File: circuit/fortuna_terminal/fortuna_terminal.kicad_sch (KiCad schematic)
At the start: 14 parts

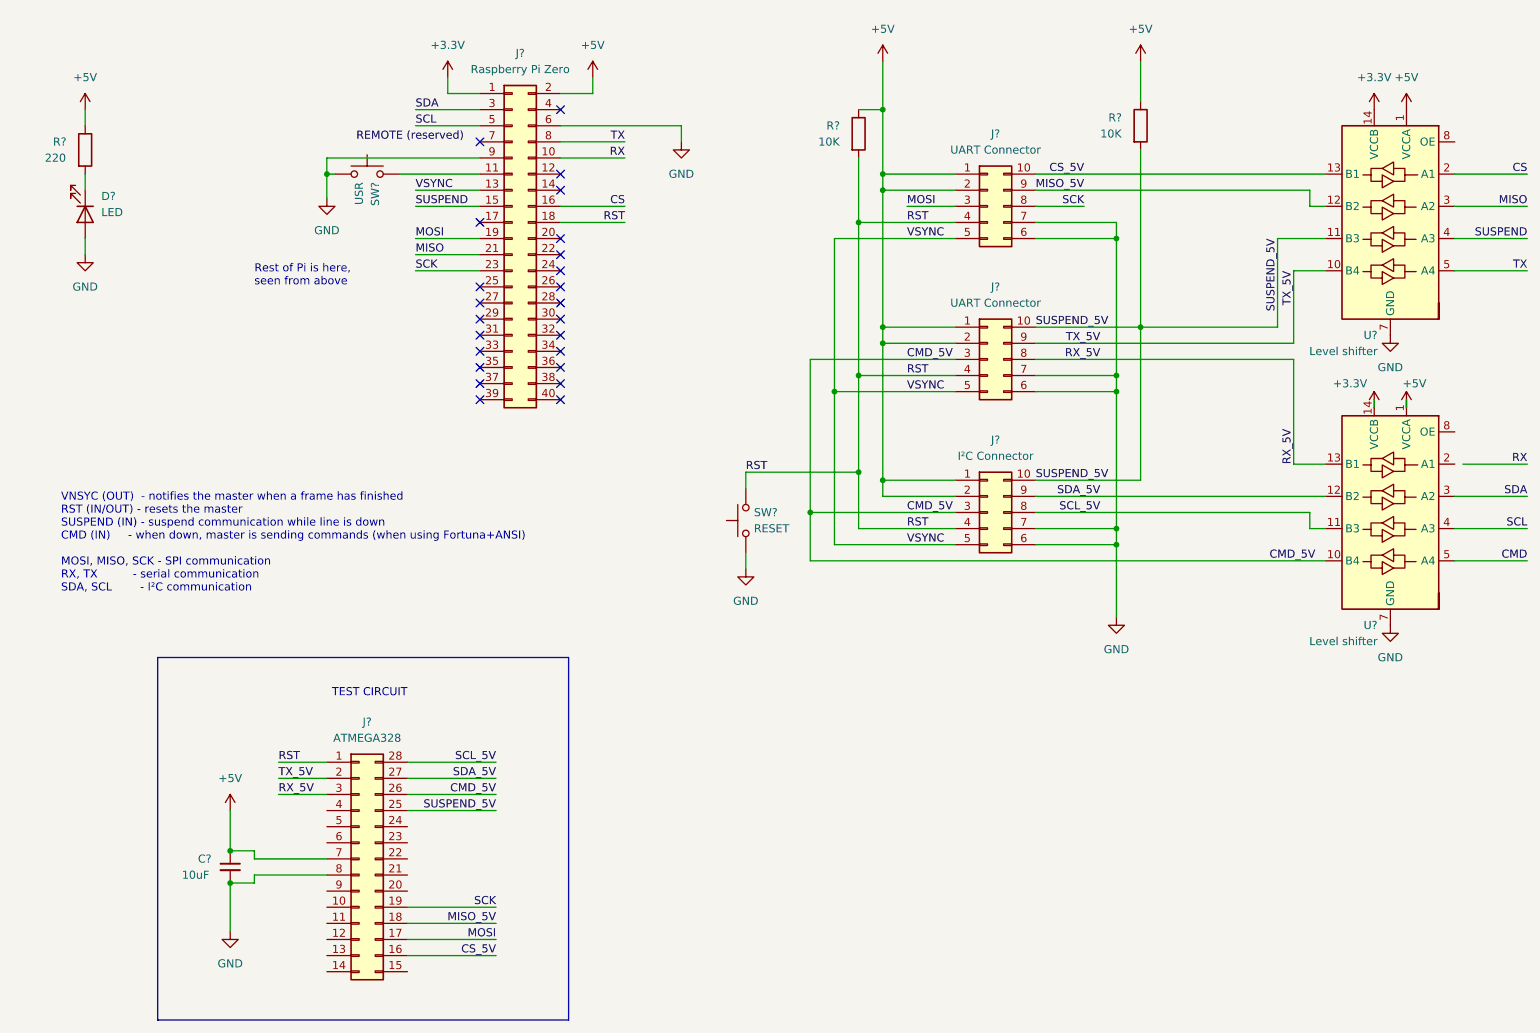
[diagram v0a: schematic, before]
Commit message: WIP
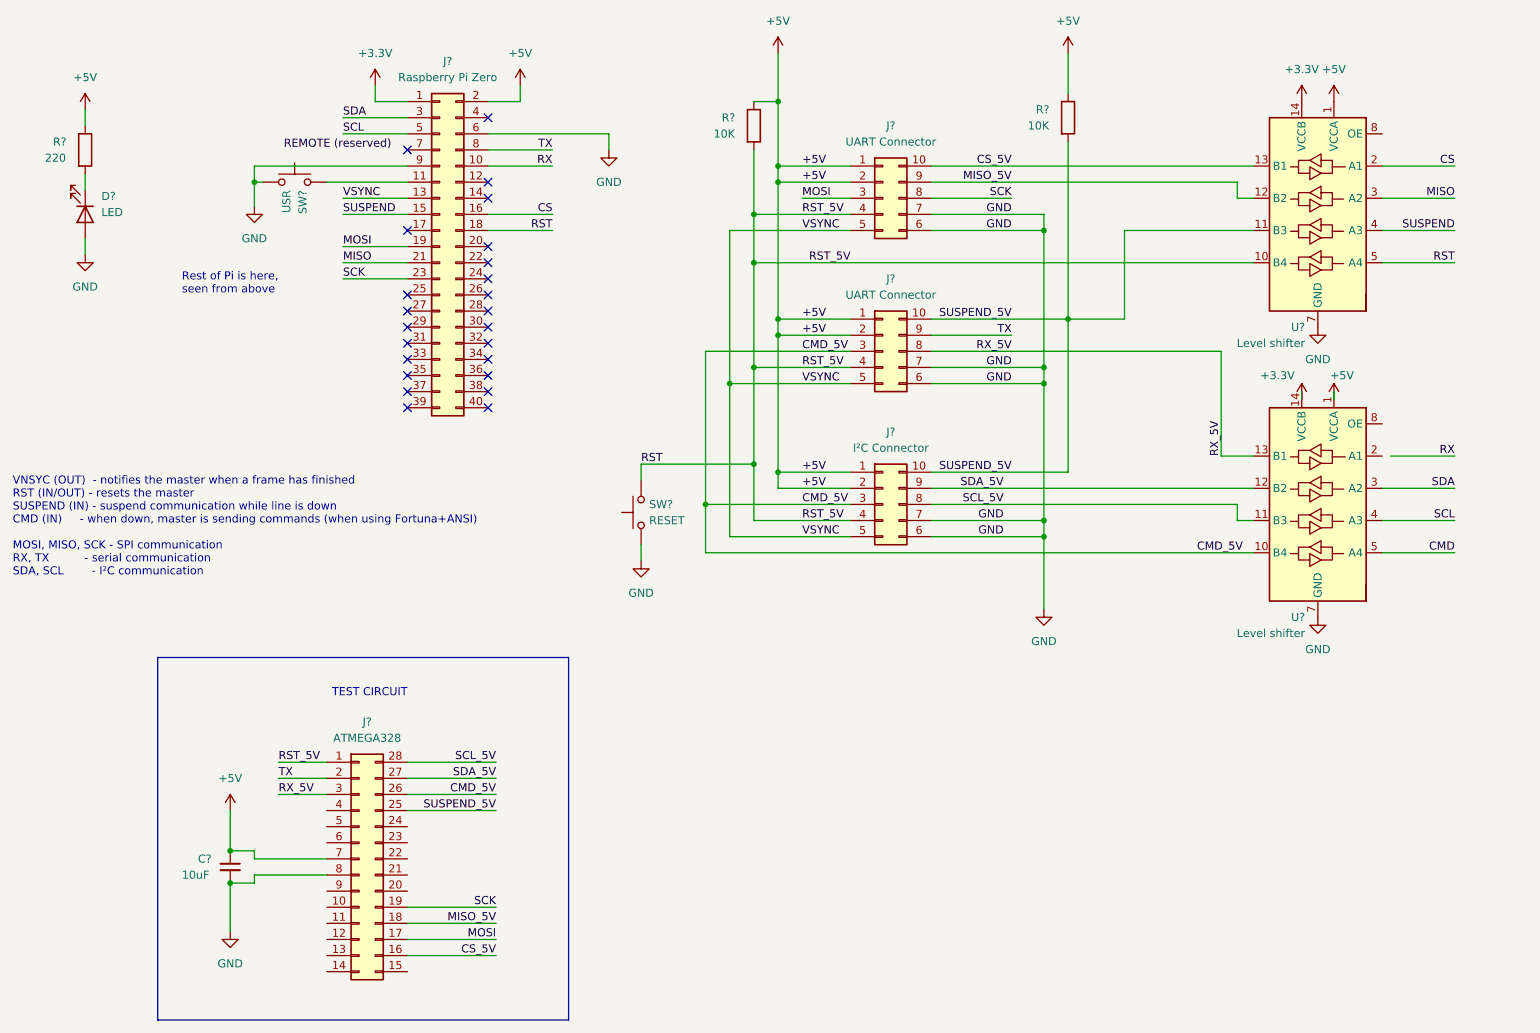
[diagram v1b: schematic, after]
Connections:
- net RST: now also U?.10 (B4), U?.5 (A4)
- net TX: now also J?.2 (Pin_2), J?.9 (Pin_9); no longer U?.5 (A4)
- removed net TX_5V: J?.2 (Pin_2), J?.9 (Pin_9), U?.10 (B4)
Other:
- moved on the sheet: J?, R?, SW?, U?
